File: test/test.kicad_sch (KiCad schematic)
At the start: 129 parts, among them SW1 MX_SW_HS, SW10 MX_SW_HS, SW11 MX_SW_HS, SW12 MX_SW_HS, SW13 MX_SW_HS, SW14 MX_SW_HS, SW15 MX_SW_HS, SW16 MX_SW_HS, SW17 MX_SW_HS, SW18 MX_SW_HS, SW19 MX_SW_HS, SW2 MX_SW_HS, SW20 MX_SW_HS, SW21 MX_SW_HS, SW22 MX_SW_HS, SW23 MX_SW_HS, SW24 MX_SW_HS, SW25 MX_SW_HS, SW26 MX_SW_HS, SW27 MX_SW_HS, SW28 MX_SW_HS, SW29 MX_SW_HS, SW3 MX_SW_HS, SW30 MX_SW_HS, SW31 MX_SW_HS, SW32 MX_SW_HS, SW33 MX_SW_HS, SW34 MX_SW_HS, SW35 MX_SW_HS, SW36 MX_SW_HS, SW37 MX_SW_HS, SW38 MX_SW_HS, SW39 MX_SW_HS, SW4 MX_SW_HS, SW40 MX_SW_HS, SW41 MX_SW_HS, SW42 MX_SW_HS, SW43 MX_SW_HS, SW44 MX_SW_HS, SW45 MX_SW_HS, SW46 MX_SW_HS, SW47 MX_SW_HS, SW48 MX_SW_HS, SW49 MX_SW_HS, SW5 MX_SW_HS, SW50 MX_SW_HS, SW51 MX_SW_HS, SW52 MX_SW_HS, SW53 MX_SW_HS, SW54 MX_SW_HS, SW55 MX_SW_HS, SW56 MX_SW_HS, SW57 MX_SW_HS, SW58 MX_SW_HS, SW59 MX_SW_HS, SW6 MX_SW_HS, SW60 MX_SW_HS, SW61 MX_SW_HS, SW62 MX_SW_HS, SW63 MX_SW_HS, SW64 MX_SW_HS, SW7 MX_SW_HS, SW8 MX_SW_HS, SW9 MX_SW_HS, U1 ProMicro

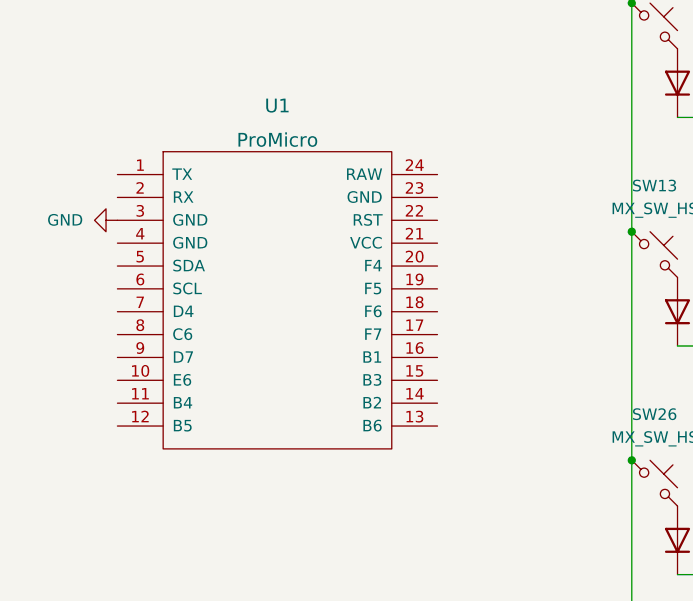
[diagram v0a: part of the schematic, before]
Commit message: fix
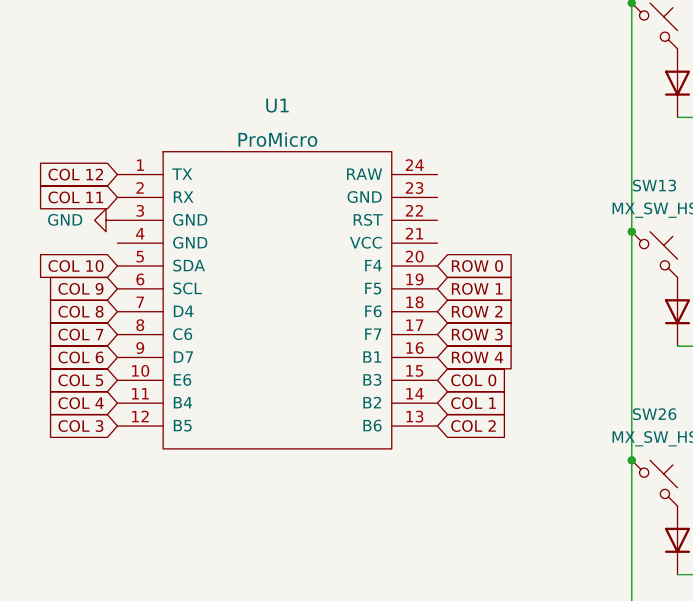
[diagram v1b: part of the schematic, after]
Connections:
- net COL 0: now also U1.15 (B3)
- net COL 1: now also U1.14 (B2)
- net COL 10: now also U1.5 (SDA)
- net COL 11: now also U1.2 (RX)
- net COL 12: now also U1.1 (TX)
- net COL 2: now also U1.13 (B6)
- net COL 3: now also U1.12 (B5)
- net COL 4: now also U1.11 (B4)
- net COL 5: now also U1.10 (E6)
- net COL 6: now also U1.9 (D7)
- net COL 7: now also U1.8 (C6)
- net COL 8: now also U1.7 (D4)
- net COL 9: now also U1.6 (SCL)
- net ROW 0: now also U1.20 (F4)
- net ROW 1: now also U1.19 (F5)
- net ROW 2: now also U1.18 (F6)
- net ROW 3: now also U1.17 (F7)
- net ROW 4: now also U1.16 (B1)
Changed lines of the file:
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@@
     (stroke (width 0) (type default) (color 0 0 0 0))
   )
+  (global_label "COL 4" (shape input) (at 20.32 88.9 180) (fields_autoplaced)
+    (effects (font (size 1.27 1.27)) (justify right))
+    (property "Intersheet References" "${INTERSHEET_REFS}" (id 0) (at 12.1012 88.8206 0)
+      (effects (font (size 1.27 1.27)) (justify right) hide)
+    )
+  )
+  (global_label "COL 2" (shape input) (at 55.88 91.44 0) (fields_autoplaced)
+    (effects (font (size 1.27 1.27)) (justify left))
+    (property "Intersheet References" "${INTERSHEET_REFS}" (id 0) (at 64.0988 91.3606 0)
+      (effects (font (size 1.27 1.27)) (justify left) hide)
+    )
+  )
   (global_label "COL 10" (shape input) (at 204.47 31.75 90) (fields_autoplaced)
     (effects (font (size 1.27 1.27)) (justify left))
@@
     )
   )
+  (global_label "ROW 3" (shape input) (at 55.88 81.28 0) (fields_autoplaced)
+    (effects (font (size 1.27 1.27)) (justify left))
+    (property "Intersheet References" "${INTERSHEET_REFS}" (id 0) (at 64.5221 81.2006 0)
+      (effects (font (size 1.27 1.27)) (justify left) hide)
+    )
+  )
   (global_label "COL 1" (shape input) (at 90.17 31.75 90) (fields_autoplaced)
     (effects (font (size 1.27 1.27)) (justify left))
@@
     )
   )
+  (global_label "COL 6" (shape input) (at 20.32 83.82 180) (fields_autoplaced)
+    (effects (font (size 1.27 1.27)) (justify right))
+    (property "Intersheet References" "${INTERSHEET_REFS}" (id 0) (at 12.1012 83.7406 0)
+      (effects (font (size 1.27 1.27)) (justify right) hide)
+    )
+  )
+  (global_label "COL 7" (shape input) (at 20.32 81.28 180) (fields_autoplaced)
+    (effects (font (size 1.27 1.27)) (justify right))
+    (property "Intersheet References" "${INTERSHEET_REFS}" (id 0) (at 12.1012 81.2006 0)
+      (effects (font (size 1.27 1.27)) (justify right) hide)
+    )
+  )
+  (global_label "ROW 1" (shape input) (at 55.88 76.2 0) (fields_autoplaced)
+    (effects (font (size 1.27 1.27)) (justify left))
+    (property "Intersheet References" "${INTERSHEET_REFS}" (id 0) (at 64.5221 76.1206 0)
+      (effects (font (size 1.27 1.27)) (justify left) hide)
+    )
+  )
   (global_label "COL 8" (shape input) (at 179.07 31.75 90) (fields_autoplaced)
     (effects (font (size 1.27 1.27)) (justify left))
@@
     )
   )
+  (global_label "ROW 4" (shape input) (at 55.88 83.82 0) (fields_autoplaced)
+    (effects (font (size 1.27 1.27)) (justify left))
+    (property "Intersheet References" "${INTERSHEET_REFS}" (id 0) (at 64.5221 83.7406 0)
+      (effects (font (size 1.27 1.27)) (justify left) hide)
+    )
+  )
+  (global_label "ROW 2" (shape input) (at 55.88 78.74 0) (fields_autoplaced)
+    (effects (font (size 1.27 1.27)) (justify left))
+    (property "Intersheet References" "${INTERSHEET_REFS}" (id 0) (at 64.5221 78.6606 0)
+      (effects (font (size 1.27 1.27)) (justify left) hide)
+    )
+  )
+  (global_label "COL 3" (shape input) (at 20.32 91.44 180) (fields_autoplaced)
+    (effects (font (size 1.27 1.27)) (justify right))
+    (property "Intersheet References" "${INTERSHEET_REFS}" (id 0) (at 12.1012 91.3606 0)
+      (effects (font (size 1.27 1.27)) (justify right) hide)
+    )
+  )
+  (global_label "COL 5" (shape input) (at 20.32 86.36 180) (fields_autoplaced)
+    (effects (font (size 1.27 1.27)) (justify right))
+    (property "Intersheet References" "${INTERSHEET_REFS}" (id 0) (at 12.1012 86.2806 0)
+      (effects (font (size 1.27 1.27)) (justify right) hide)
+    )
+  )
+  (global_label "COL 8" (shape input) (at 20.32 78.74 180) (fields_autoplaced)
+    (effects (font (size 1.27 1.27)) (justify right))
+    (property "Intersheet References" "${INTERSHEET_REFS}" (id 0) (at 12.1012 78.6606 0)
+      (effects (font (size 1.27 1.27)) (justify right) hide)
+    )
+  )
   (global_label "COL 6" (shape input) (at 153.67 31.75 90) (fields_autoplaced)
     (effects (font (size 1.27 1.27)) (justify left))
@@
     )
   )
+  (global_label "COL 0" (shape input) (at 55.88 86.36 0) (fields_autoplaced)
+    (effects (font (size 1.27 1.27)) (justify left))
+    (property "Intersheet References" "${INTERSHEET_REFS}" (id 0) (at 64.0988 86.2806 0)
+      (effects (font (size 1.27 1.27)) (justify left) hide)
+    )
+  )
   (global_label "ROW 0" (shape input) (at 255.27 57.15 0) (fields_autoplaced)
     (effects (font (size 1.27 1.27)) (justify left))
@@
     )
   )
+  (global_label "COL 12" (shape input) (at 20.32 63.5 180) (fields_autoplaced)
+    (effects (font (size 1.27 1.27)) (justify right))
+    (property "Intersheet References" "${INTERSHEET_REFS}" (id 0) (at 10.8917 63.4206 0)
+      (effects (font (size 1.27 1.27)) (justify right) hide)
+    )
+  )
+  (global_label "ROW 0" (shape input) (at 55.88 73.66 0) (fields_autoplaced)
+    (effects (font (size 1.27 1.27)) (justify left))
+    (property "Intersheet References" "${INTERSHEET_REFS}" (id 0) (at 64.5221 73.5806 0)
+      (effects (font (size 1.27 1.27)) (justify left) hide)
+    )
+  )
+  (global_label "COL 1" (shape input) (at 55.88 88.9 0) (fields_autoplaced)
+    (effects (font (size 1.27 1.27)) (justify left))
+    (property "Intersheet References" "${INTERSHEET_REFS}" (id 0) (at 64.0988 88.8206 0)
+      (effects (font (size 1.27 1.27)) (justify left) hide)
+    )
+  )
+  (global_label "COL 11" (shape input) (at 20.32 66.04 180) (fields_autoplaced)
+    (effects (font (size 1.27 1.27)) (justify right))
+    (property "Intersheet References" "${INTERSHEET_REFS}" (id 0) (at 10.8917 65.9606 0)
+      (effects (font (size 1.27 1.27)) (justify right) hide)
+    )
+  )
   (global_label "ROW 1" (shape input) (at 255.27 82.55 0) (fields_autoplaced)
     (effects (font (size 1.27 1.27)) (justify left))
@@
     )
   )
+  (global_label "COL 10" (shape input) (at 20.32 73.66 180) (fields_autoplaced)
+    (effects (font (size 1.27 1.27)) (justify right))
+    (property "Intersheet References" "${INTERSHEET_REFS}" (id 0) (at 10.8917 73.5806 0)
+      (effects (font (size 1.27 1.27)) (justify right) hide)
+    )
+  )
   (global_label "COL 2" (shape input) (at 102.87 31.75 90) (fields_autoplaced)
     (effects (font (size 1.27 1.27)) (justify left))
@@
     )
   )
+  (global_label "COL 9" (shape input) (at 20.32 76.2 180) (fields_autoplaced)
+    (effects (font (size 1.27 1.27)) (justify right))
+    (property "Intersheet References" "${INTERSHEET_REFS}" (id 0) (at 12.1012 76.1206 0)
+      (effects (font (size 1.27 1.27)) (justify right) hide)
+    )
+  )
